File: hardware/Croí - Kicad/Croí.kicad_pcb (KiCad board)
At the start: 4 copper layers, 60 x 60 mm, 38 parts, among them J1 JTAG-10 PIN, J2 XT30PW-M, J3 ESQ-110-14-G-D, Q1 IPP060N06N, U1 W25Q128JVS, U2 ADXL375BCCZ, U3 STM32F072C8Tx, U4 BME680, U5 BMP390, U7 TLV70433DBVT, U8 TJA1051T-3, U9 LSM6DSO32TR

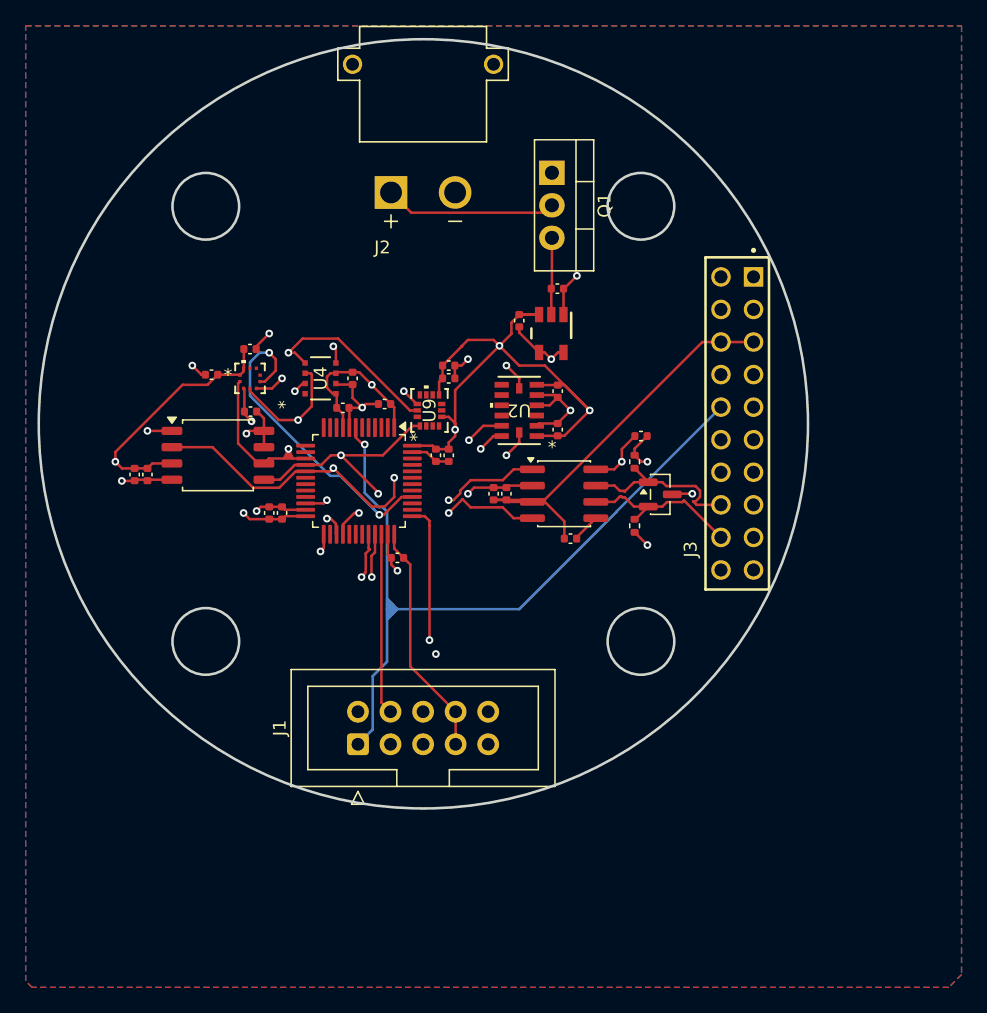
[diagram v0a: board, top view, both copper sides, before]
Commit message: minor changes
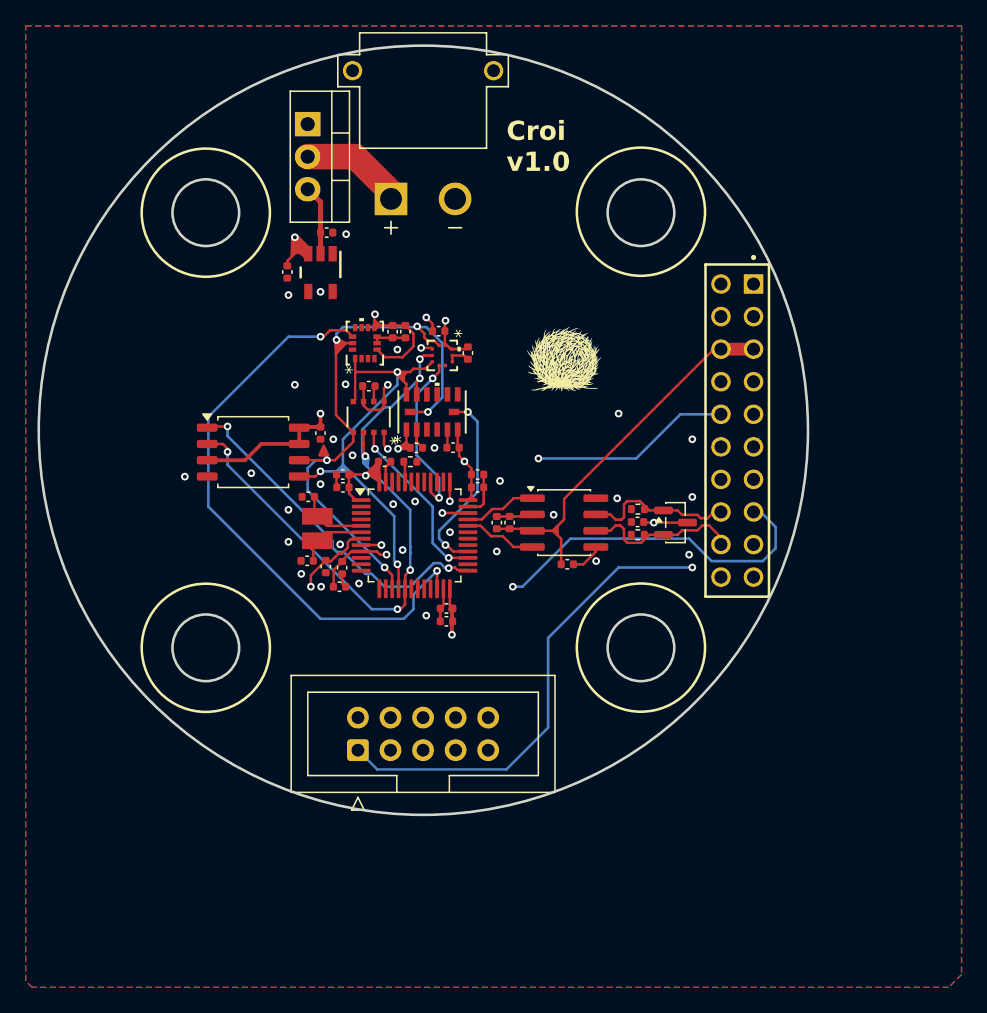
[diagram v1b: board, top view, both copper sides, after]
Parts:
- added C13: 100nF, Capacitor_SMD:C_0402_1005Metric, F.Cu at (34.4, 53.2)
- added C27: 8pF, Capacitor_SMD:C_0402_1005Metric, F.Cu at (33.0, 47.7)
- added C28: 8pF, Capacitor_SMD:C_0402_1005Metric, F.Cu at (33.0, 52.7)
- added G***: LOGO, LOGO, F.Cu at (53.0, 37.0)
- added R1: 10KΩ, Resistor_SMD:R_0402_1005Metric, F.Cu at (41.0, 45.0)
- added XTAL1: NX3225GD-8MHZ-STD-CRA-3, footprints2:XTAL_NX3225GD-8MHZ-STD-CRA-3_NDK, F.Cu at (33.8, 50.2)
- R6, R7: value 60 Ω -> 60Ω
- moved Q1 19.4 mm to (33.0, 18.7)
- moved U7 18.6 mm to (34.0, 30.2)
- moved C21 18.5 mm to (34.5, 27.1)
- moved C7 18.5 mm to (43.8, 57.4), turned to 180 degrees
- moved C23 18.5 mm to (31.4, 30.2)
- moved C18 18.0 mm to (43.2, 34.8)
- moved C12 17.7 mm to (35.7, 53.3)
- moved C10 17.3 mm to (35.5, 54.8), turned to 0 degrees
- moved C20 17.0 mm to (45.5, 36.5), turned to -90 degrees
- moved U5 15.1 mm to (43.5, 36.7), turned to -90 degrees
- moved C8 14.8 mm to (43.8, 56.4), turned to 180 degrees
- moved C3 11.1 mm to (41.5, 43.9), turned to 0 degrees
- moved C1 9.27 mm to (44.3, 43.9), turned to 180 degrees
- moved C6 7.57 mm to (39.0, 45.0), turned to 0 degrees
- moved U9 7.28 mm to (37.5, 35.8)
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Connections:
- J1 pad 2: SWCLK -> SWCLK2
- J3 pad 10: NRST -> SWCLK2
- J3 pad 17: SWCLK -> NRST
- U3 pad 26: Mode_sel -> unconnected-(U3-PB13-Pad26)
- U3 pad 37: SWCLK -> SWCLK2
- U3 pad 44: unconnected-(U3-BOOT0-Pad44) -> Net-(U3-BOOT0)
- U3 pad 5: unconnected-(U3-PF0-Pad5) -> Net-(U3-PF0)
- U3 pad 6: unconnected-(U3-PF1-Pad6) -> Net-(U3-PF1)
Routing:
- net SWCLK2: track 0.00 -> 48.4 mm, vias 0 -> 2
- net SWDIO: track 14.1 -> 55.3 mm, vias 0 -> 2
- net GND: track 65.4 -> 30.4 mm, vias 15 -> 36
- net IMU_CS: track 15.4 -> 46.3 mm
- net CAN-: track 24.5 -> 5.71 mm, vias 2 -> 0
- net SWCLK: track 18.7 -> 0.00 mm, vias 1 -> 0
- net CAN+: track 23.9 -> 5.71 mm, vias 2 -> 0
- net SPI_MISO: track 48.2 -> 36.6 mm, vias 5 -> 3
- net Net-(C26-Pad1): track 11.4 -> 0.00 mm, vias 2 -> 0
- net BMP390_CS: track 24.7 -> 13.4 mm
- net ACCELEROMETER_CS: track 25.9 -> 15.2 mm
- net 3.3V: track 160.3 -> 150.0 mm, vias 7 -> 11
- net SPICLK: track 57.4 -> 47.4 mm, vias 3 -> 5
- net Flash_CS: track 20.7 -> 27.4 mm
- net Net-(Q1-D): track 13.4 -> 7.66 mm
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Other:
- board text added: "Croi v1.0"
